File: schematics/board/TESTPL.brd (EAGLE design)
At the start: 136 x 60 mm, 31 parts

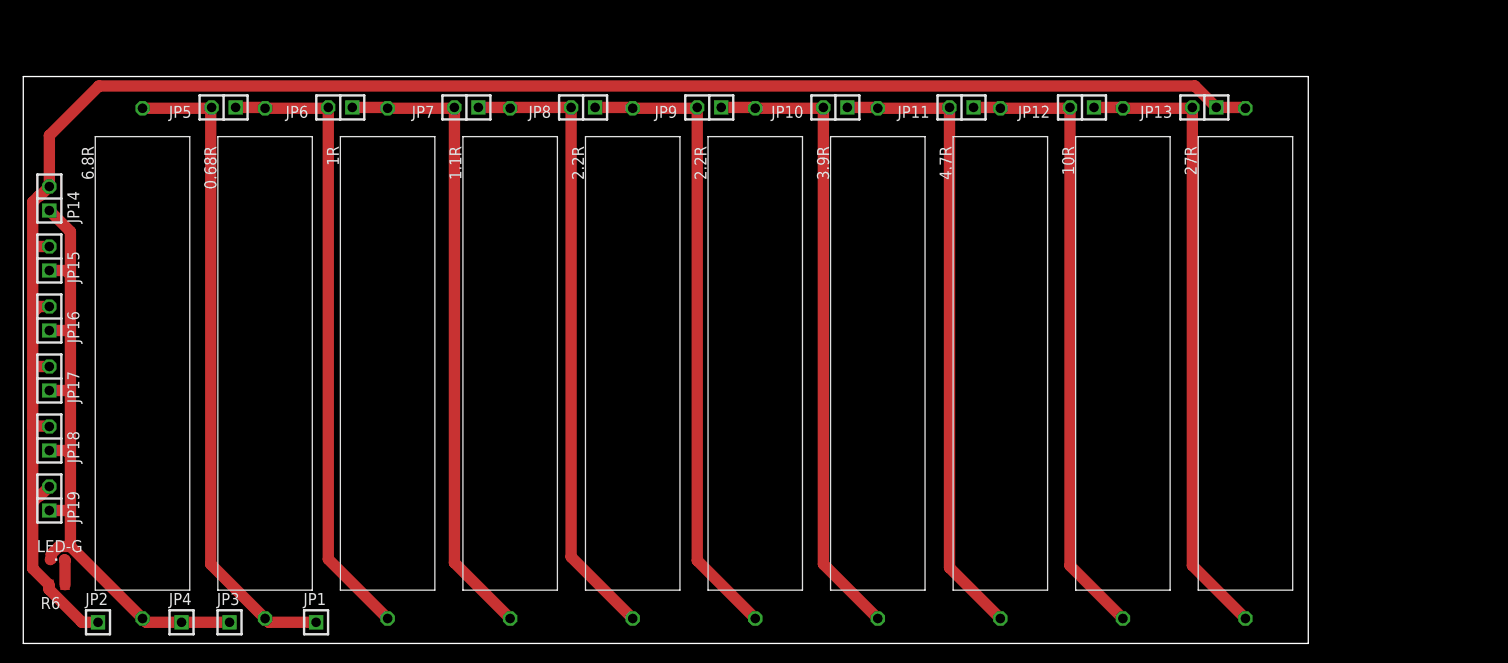
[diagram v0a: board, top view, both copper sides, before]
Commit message: Исправлена плата TESTPL
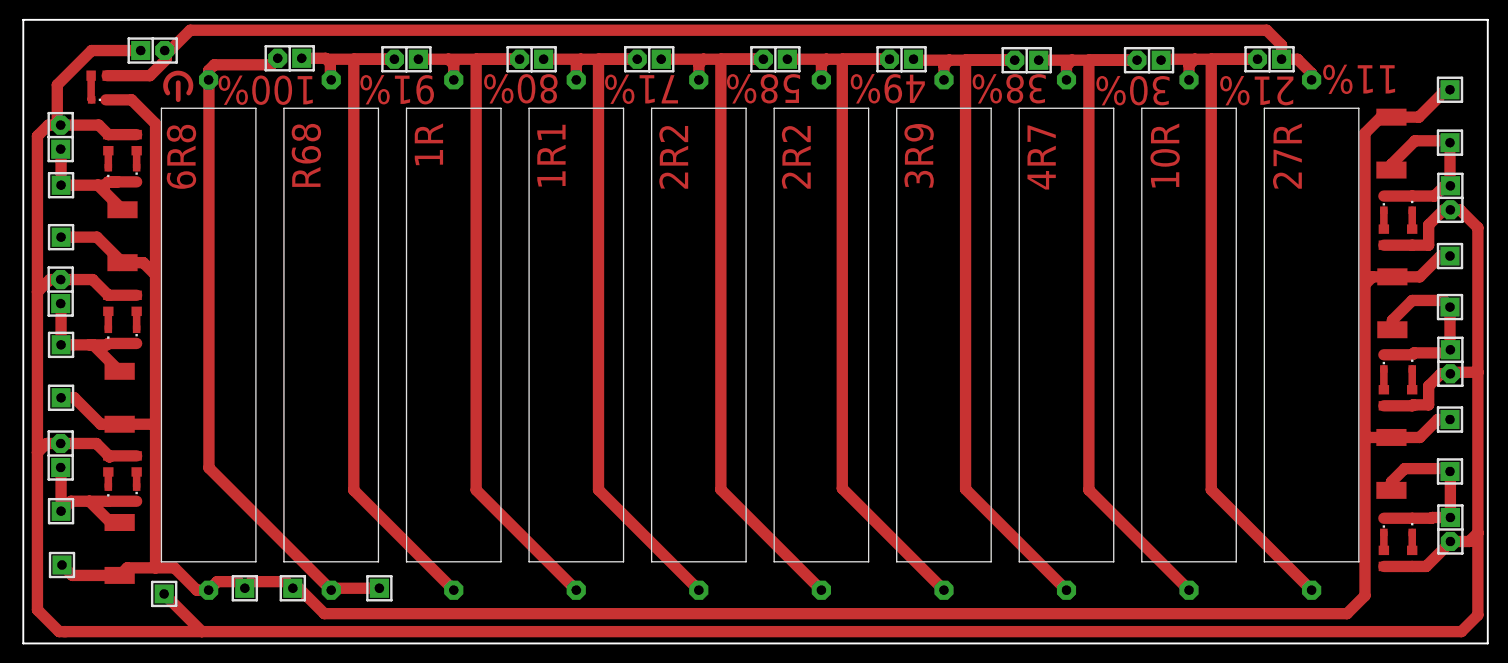
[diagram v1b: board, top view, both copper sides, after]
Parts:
- removed LED-G: (no value), led:CHIPLED_0603
- added JP20, JP21, JP22, JP23, JP24, JP25, JP26, JP27, JP28, JP29, JP30, JP31: (no value), pinheadCS:1X01
- added JP32: (no value), pinheadCS:1X02
- added LED, LED-G1, LED-G10, LED-G11, LED-G12, LED-G2, LED-G3, LED-G4, LED-G5, LED-G6, LED-G7, LED-G8, LED-G9: (no value), led:CHIPLED_0603
- added R1, R2, R3, R4, R5, R7: R100, rcl:R2512
- added R10, R11, R12, R13, R14, R15, R16, R17, R18, R19, R8, R9: 2k7, resistor:R0603
- U$1: value 6.8R -> 6R8
- U$2: value 0.68R -> R68
- U$4: value 1.1R -> 1R1
- U$5, U$6: value 2.2R -> 2R2
- U$7: value 3.9R -> 3R9
- U$8: value 4.7R -> 4R7
- moved JP19 151.7 mm to (151.0, 47.2), turned to 270 degrees
- moved JP17 149.1 mm to (151.0, 12.1), turned to 270 degrees
- moved JP18 148.5 mm to (151.0, 29.8), turned to 270 degrees
- moved R6 54.1 mm to (8.03, 60.1), turned to 180 degrees
- moved JP16 14.5 mm to (3.96, 19.9)
- moved JP5 8.72 mm to (28.2, 61.9)
- moved JP12 8.68 mm to (119.2, 61.7)
- moved JP10 8.66 mm to (93.0, 61.8)
- moved JP6 8.66 mm to (40.5, 61.8)
- moved JP8 8.66 mm to (66.2, 61.8)
- moved JP9 8.66 mm to (79.6, 61.8)
- moved JP13 8.58 mm to (131.9, 61.8)
- moved JP7 8.58 mm to (53.8, 61.8)
- moved JP11 8.52 mm to (106.2, 61.7)
- moved U$2 7.62 mm to (32.6, 32.6)
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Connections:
- new net GND: JP21.1, JP23.1, JP25.1, JP27.1, JP29.1, JP3.1, JP31.1, JP4.1, LED.C, R1.1, R2.1, R3.1, R4.1, R5.1, R7.1, U$1.P$2
- new net N$12: JP19.1, JP28.1, LED-G11.A, LED-G5.C, R5.2
- new net N$13: JP18.1, JP26.1, LED-G10.A, LED-G4.C, R4.2
- new net N$14: JP14.1, JP24.1, LED-G3.C, LED-G9.A, R3.2
- new net N$15: JP15.1, JP22.1, LED-G2.C, LED-G8.A, R2.2
- new net N$16: JP16.1, JP20.1, LED-G1.C, LED-G7.A, R1.2
- new net N$17: JP13.1, JP32.2, R6.1, U$10.P$1
- new net N$18: LED-G1.A, R8.2
- new net N$19: LED-G2.A, R9.2
- new net N$20: LED-G3.A, R10.2
- new net N$21: LED-G4.A, R11.2
- new net N$22: LED-G5.A, R12.2
- new net N$23: LED-G6.A, R13.2
- new net N$24: LED-G8.C, R15.1
- new net N$25: LED-G7.C, R14.1
- new net N$26: LED-G9.C, R16.1
- new net N$27: LED-G10.C, R17.1
- new net N$28: LED-G11.C, R18.1
- new net N$29: LED-G12.C, R19.1
- net N$10: now also JP30.1, LED-G12.A, LED-G6.C, R7.2; no longer JP14.1, JP15.1, JP16.1, JP18.1, JP19.1, JP3.1, JP4.1, LED-G.C, U$1.P$2
- net N$11: now also JP32.1, R10.1, R11.1, R12.1, R13.1, R14.2, R15.2, R16.2, R17.2, R18.2, R19.2, R8.1, R9.1; no longer JP13.1, R6.1, U$10.P$1
- net N$38: now also LED.A; no longer LED-G.A
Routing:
- net GND: track 0.00 -> 299.3 mm
- net N$11: track 195.8 -> 338.4 mm
- net N$17: track 0.00 -> 133.7 mm
- net N$10: track 71.3 -> 20.0 mm
- net N$13: track 0.00 -> 20.1 mm
- net N$12: track 0.00 -> 20.0 mm
- net N$16: track 0.00 -> 17.2 mm
- net N$14: track 0.00 -> 16.7 mm
- net N$15: track 0.00 -> 16.4 mm
- net N$8: track 66.7 -> 78.3 mm
- net N$7: track 67.2 -> 78.8 mm
- net N$6: track 67.4 -> 78.9 mm
- net N$9: track 66.9 -> 78.2 mm
- net N$3: track 67.4 -> 78.3 mm
- net N$5: track 67.5 -> 78.3 mm
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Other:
- board size 136 x 60 mm -> 155 x 66 mm
- board text added: "100%"
- board text added: "11%"
- board text added: "21%"
- board text added: "30%"
- board text added: "38%"
- board text added: "49%"
- board text added: "58%"
- board text added: "71%"
- board text added: "80%"
- board text added: "91%"

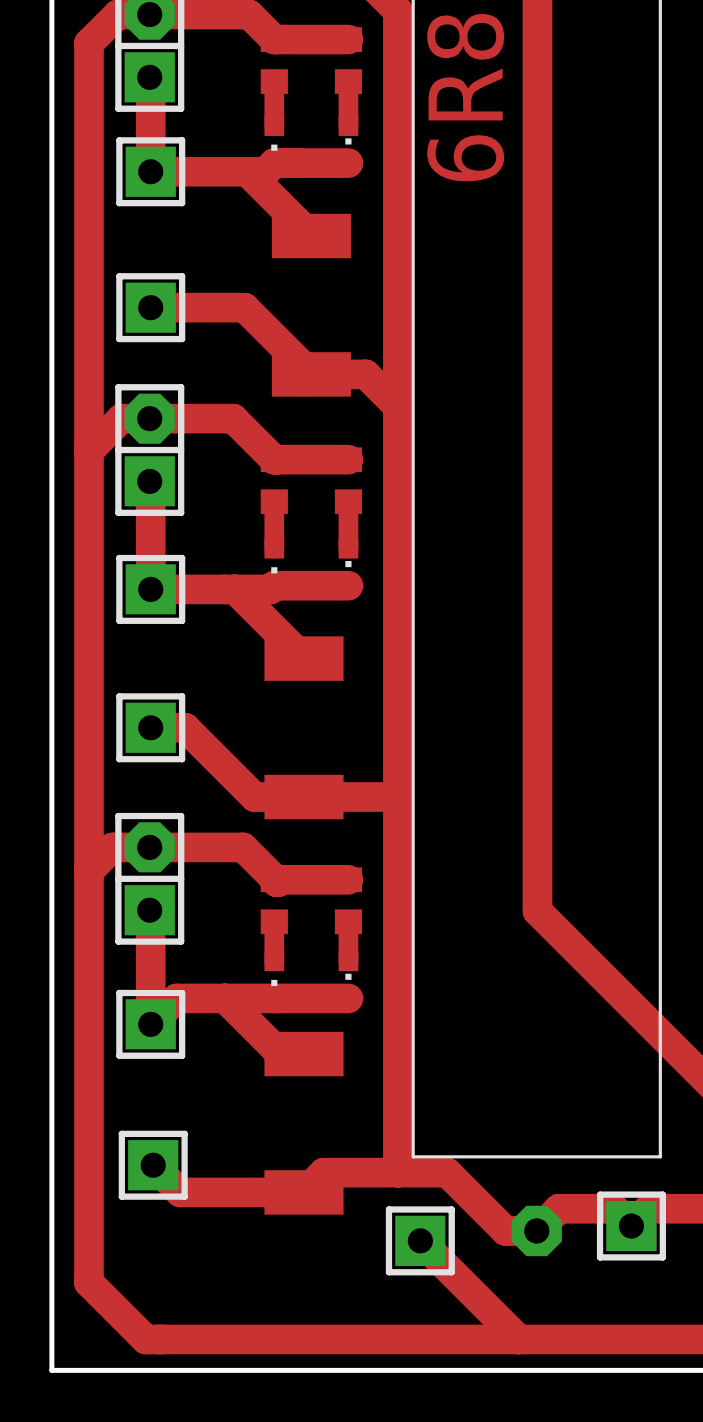
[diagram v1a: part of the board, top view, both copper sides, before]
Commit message: Незначительные изменения TESTPL
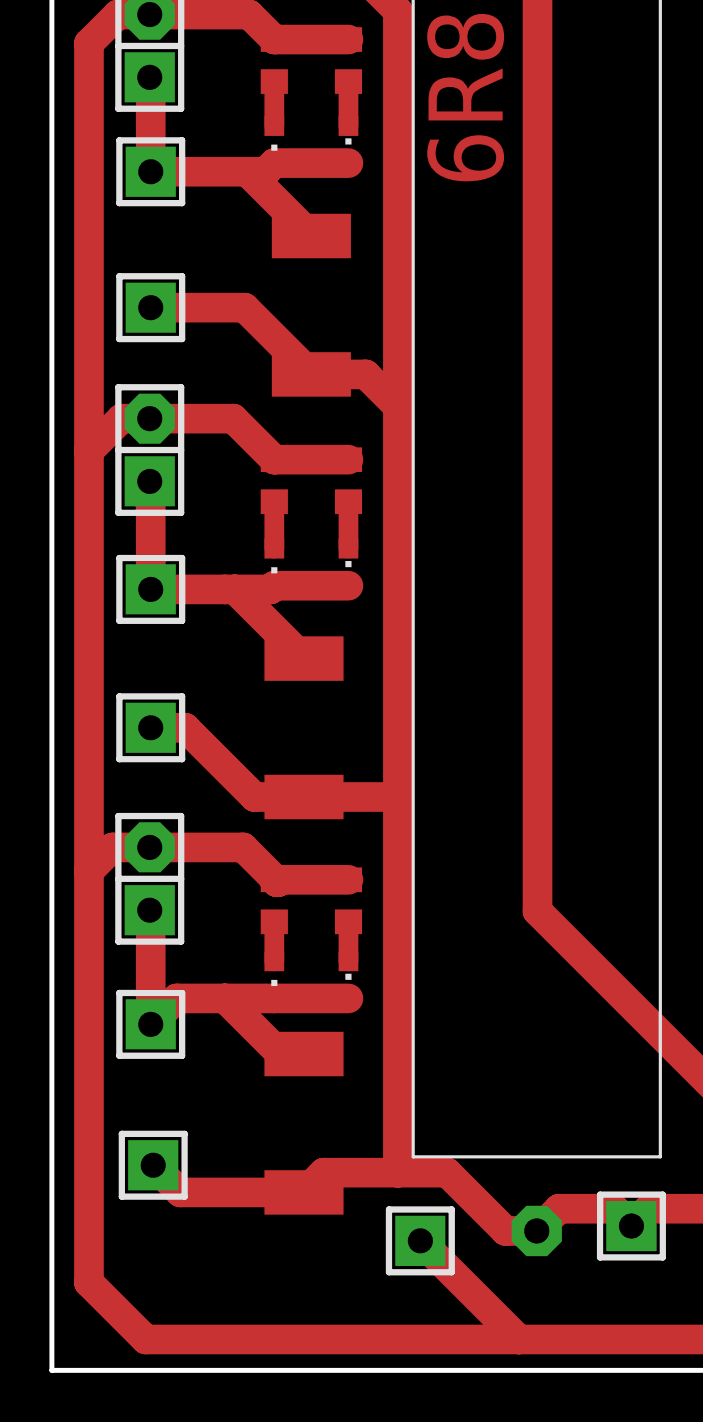
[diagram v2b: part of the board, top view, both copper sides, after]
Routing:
- net N$14: track 16.7 -> 15.7 mm
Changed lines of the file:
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@@
 <contactref element="JP27" pad="1"/>
 <contactref element="JP29" pad="1"/>
-<wire x1="10.5" y1="40.3" x2="10.2" y2="40" width="1.2" layer="1"/>
 <wire x1="8.2" y1="23.2" x2="10.2" y2="23.2" width="1.2" layer="1"/>
 <wire x1="19.62" y1="5.64" x2="18.36" y2="5.64" width="1.2" layer="1"/>
@@
 <wire x1="3.96" y1="52.32" x2="4" y2="52.28" width="1.2" layer="1"/>
 <wire x1="4" y1="52.28" x2="4" y2="48.5" width="1.2" layer="1"/>
-<wire x1="10" y1="48.85" x2="9" y2="48.85" width="1.2" layer="1"/>
 <wire x1="4" y1="48.5" x2="7.9" y2="48.5" width="1.2" layer="1"/>
 <wire x1="7.9" y1="48.5" x2="8.65" y2="48.5" width="1.2" layer="1"/>
@@
 <wire x1="1.5" y1="37.2" x2="2.81" y2="38.51" width="1.2" layer="1"/>
 <wire x1="2.81" y1="38.51" x2="3.96" y2="38.51" width="1.2" layer="1"/>
-<wire x1="9.09325625" y1="36.85" x2="9" y2="36.85" width="1.2" layer="1"/>
 <wire x1="9" y1="36.85" x2="12" y2="36.85" width="1.2" layer="1"/>
 <wire x1="1.5" y1="20.2" x2="2.46" y2="21.16" width="1.2" layer="1"/>
@@
 <wire x1="18.9" y1="1.25" x2="14.91" y2="5.24" width="1.2" layer="1"/>
 <wire x1="152.2" y1="1.25" x2="18.9" y2="1.25" width="1.2" layer="1"/>
-<wire x1="4.52" y1="1.25" x2="3.8" y2="1.25" width="1.2" layer="1"/>
-<wire x1="3.8" y1="1.25" x2="1.5" y2="3.55" width="1.2" layer="1"/>
 <wire x1="1.5" y1="3.55" x2="1.5" y2="20.2" width="1.2" layer="1"/>
-<wire x1="18.9" y1="1.25" x2="4.26" y2="1.25" width="1.2" layer="1"/>
 <wire x1="153.95" y1="11.7" x2="153.95" y2="28.7" width="1.2" layer="1"/>
 <wire x1="3.96" y1="38.51" x2="7.34" y2="38.51" width="1.2" layer="1"/>
@@
 <wire x1="7.99" y1="54.86" x2="9" y2="53.85" width="1.2" layer="1"/>
 <wire x1="9" y1="53.85" x2="12" y2="53.85" width="1.2" layer="1"/>
-<wire x1="4.26" y1="1.25" x2="4.52" y2="1.25" width="0" layer="19" extent="1-1"/>
+<wire x1="3.8" y1="1.25" x2="1.5" y2="3.55" width="1.2" layer="1"/>
+<wire x1="18.9" y1="1.25" x2="3.8" y2="1.25" width="1.2" layer="1"/>
 </signal>
 <signal name="N$17">
